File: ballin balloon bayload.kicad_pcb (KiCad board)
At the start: 4 copper layers, 73 x 86 mm, 13 parts, among them J1 Molex 0510211000, J2 Molex 0532611071, J3 Molex 0510211000, J4 Conn_01x06_Pin, J5 Conn_01x06_Pin, U1 MICROSD_SPI_OR_SDIO_CARD, U2 3073, U3 2472

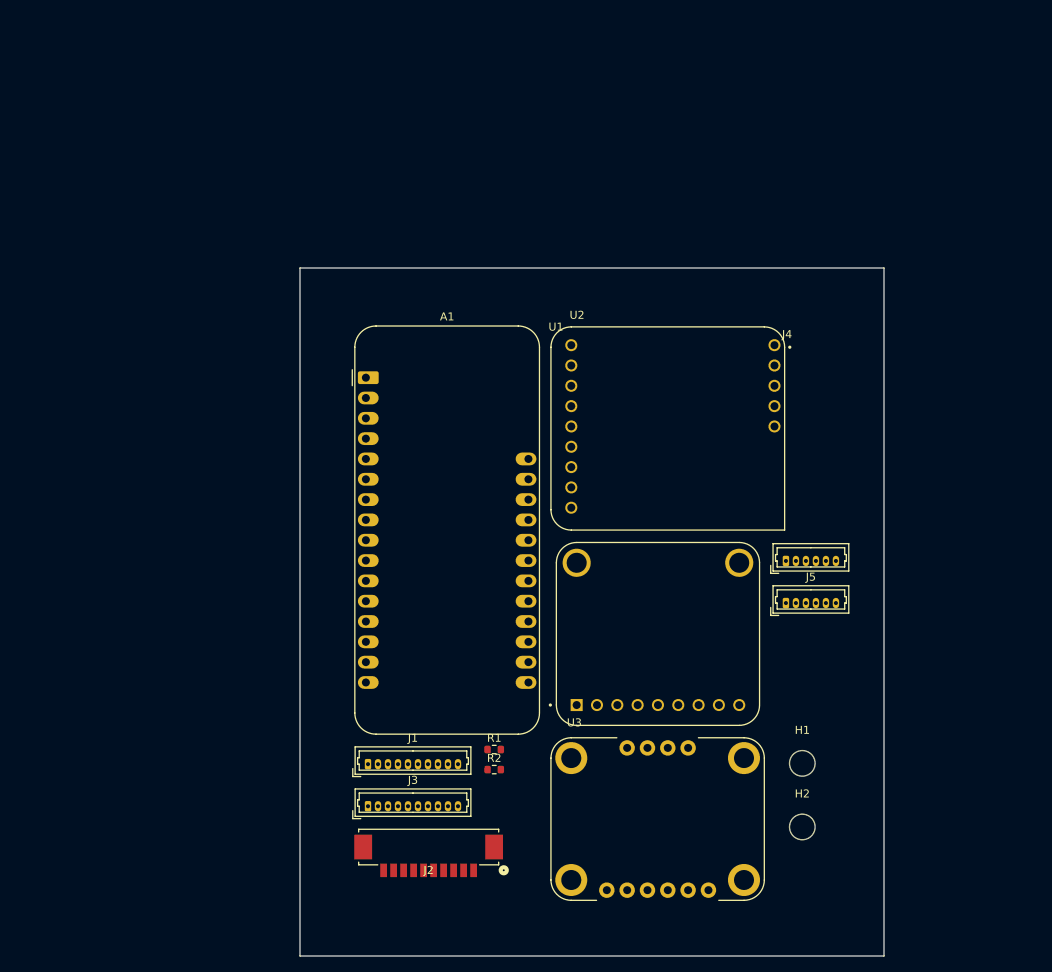
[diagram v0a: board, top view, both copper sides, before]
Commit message: "finished breakout version"
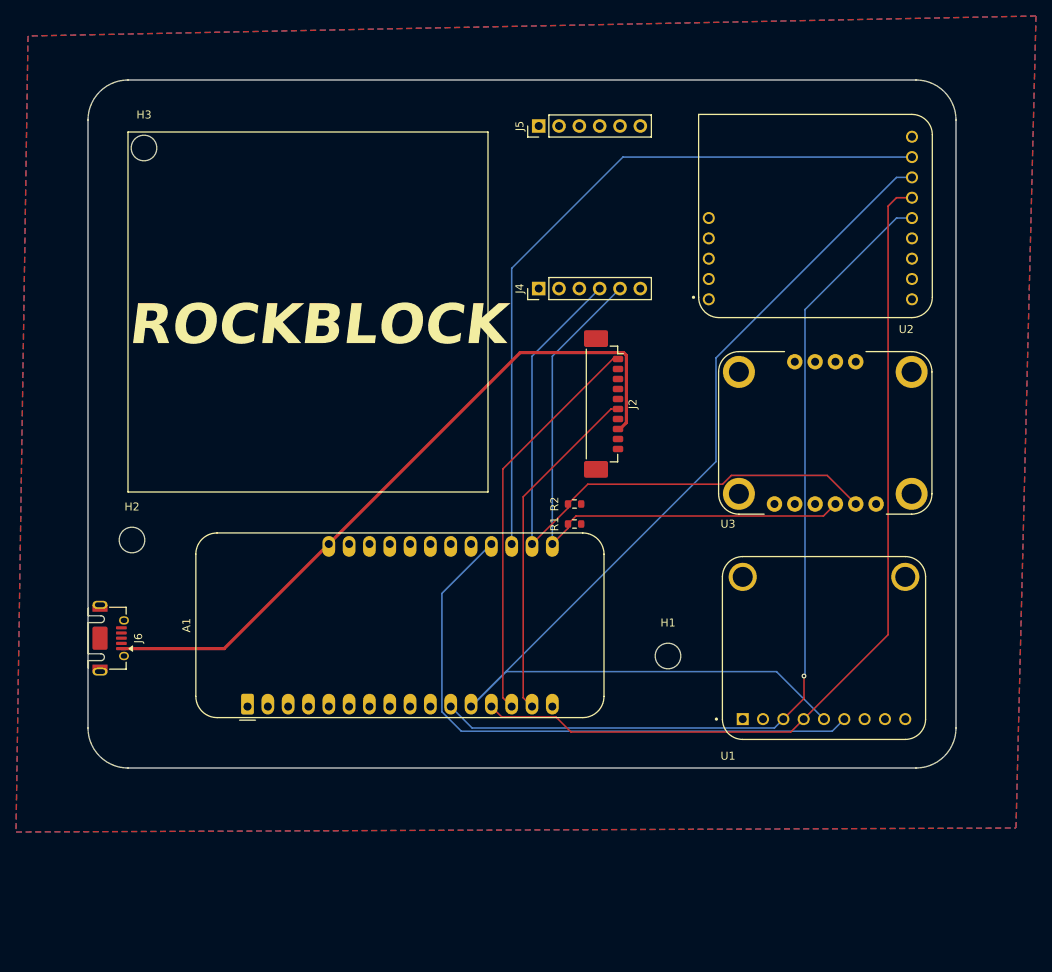
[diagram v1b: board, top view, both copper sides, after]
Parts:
- removed J1, J3: Molex 0510211000, Connector_Molex:Molex_PicoBlade_53047-1010_1x10_P1.25mm_Vertical
- added H3: rockblock, MountingHole:MountingHole_3.2mm_M3, F.Cu at (45.5, 74.5)
- added J6: USB_B_Micro, Connector_USB:USB_Micro-AB_Molex_47590-0001, F.Cu at (39.6, 135.8)
- J2: footprint footprints-extra:CONN_532610001-SD_10_MOL -> Connector_Molex:Molex_PicoBlade_53398-1071_1x10-1MP_P1.25mm_Vertical
- J4, J5: footprint Connector_Molex:Molex_PicoBlade_53047-0610_1x06_P1.25mm_Vertical -> Connector_PinHeader_2.54mm:PinHeader_1x06_P2.54mm_Vertical
- moved H2 91.1 mm to (44.0, 123.5)
- moved J5 67.2 mm to (94.8, 71.8), turned to 90 degrees
- moved J2 59.7 mm to (103.5, 106.5), turned to -90 degrees
- moved U3 52.6 mm to (130.7, 110.1)
- moved J4 46.0 mm to (94.8, 92.1), turned to 90 degrees
- moved A1 43.7 mm to (58.4, 144.3), turned to 90 degrees
- moved R2 34.7 mm to (99.3, 119.0), turned to 180 degrees
- moved U2 32.3 mm to (129.4, 83.0), turned to 180 degrees
- moved R1 29.9 mm to (99.3, 121.5), turned to 180 degrees
- moved H1 21.5 mm to (111.0, 138.0)
- moved U1 20.8 mm to (130.5, 137.0)
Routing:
- net /inside/MOSI: track 0.00 -> 138.5 mm
- net /inside/SCK: track 0.00 -> 113.6 mm, vias 0 -> 1
- net /inside/MISO: track 0.00 -> 112.9 mm
- net /inside/CS_LoRa: track 0.00 -> 91.2 mm
- net +5V: track 0.00 -> 88.4 mm
- net /inside/SCL: track 0.00 -> 81.2 mm
- net /inside/CS_microSD: track 0.00 -> 75.5 mm
- net /inside/SDA: track 0.00 -> 73.2 mm
- net /inside/RX_MCU: track 0.00 -> 50.2 mm
- net /inside/TX_MCU: track 0.00 -> 43.1 mm
- added copper zone on In1.Cu, net +3V3
- added copper zone on B.Cu, net GND
- added copper zone on F.Cu, net GND
- added copper zone on In2.Cu, net GND
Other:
- board size 73 x 86 mm -> 108.5 x 86 mm
- board text added: "ROCKBLOCK"
